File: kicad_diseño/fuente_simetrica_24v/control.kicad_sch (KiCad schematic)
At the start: 6 parts, among them J4 Conn_01x04_Socket, SW1 SW_Push, SW2 SW_Push, U6 ESP32-WROOM-32E, U7 AMS1117-3.3

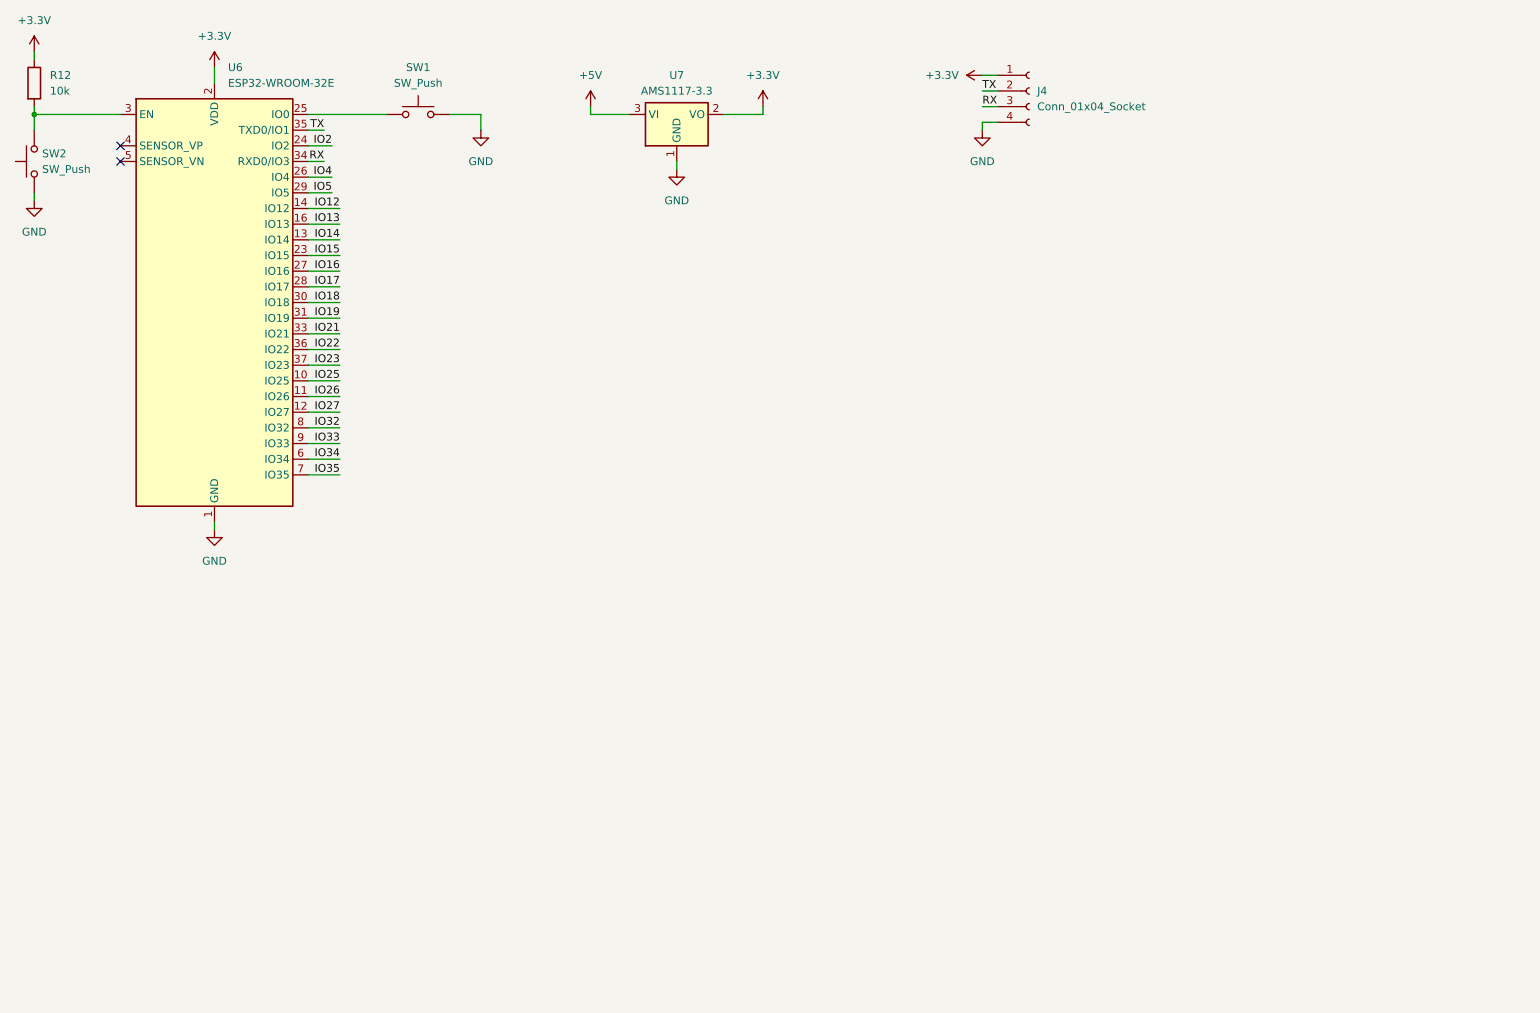
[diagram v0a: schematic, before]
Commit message: Update Fte - Pcb
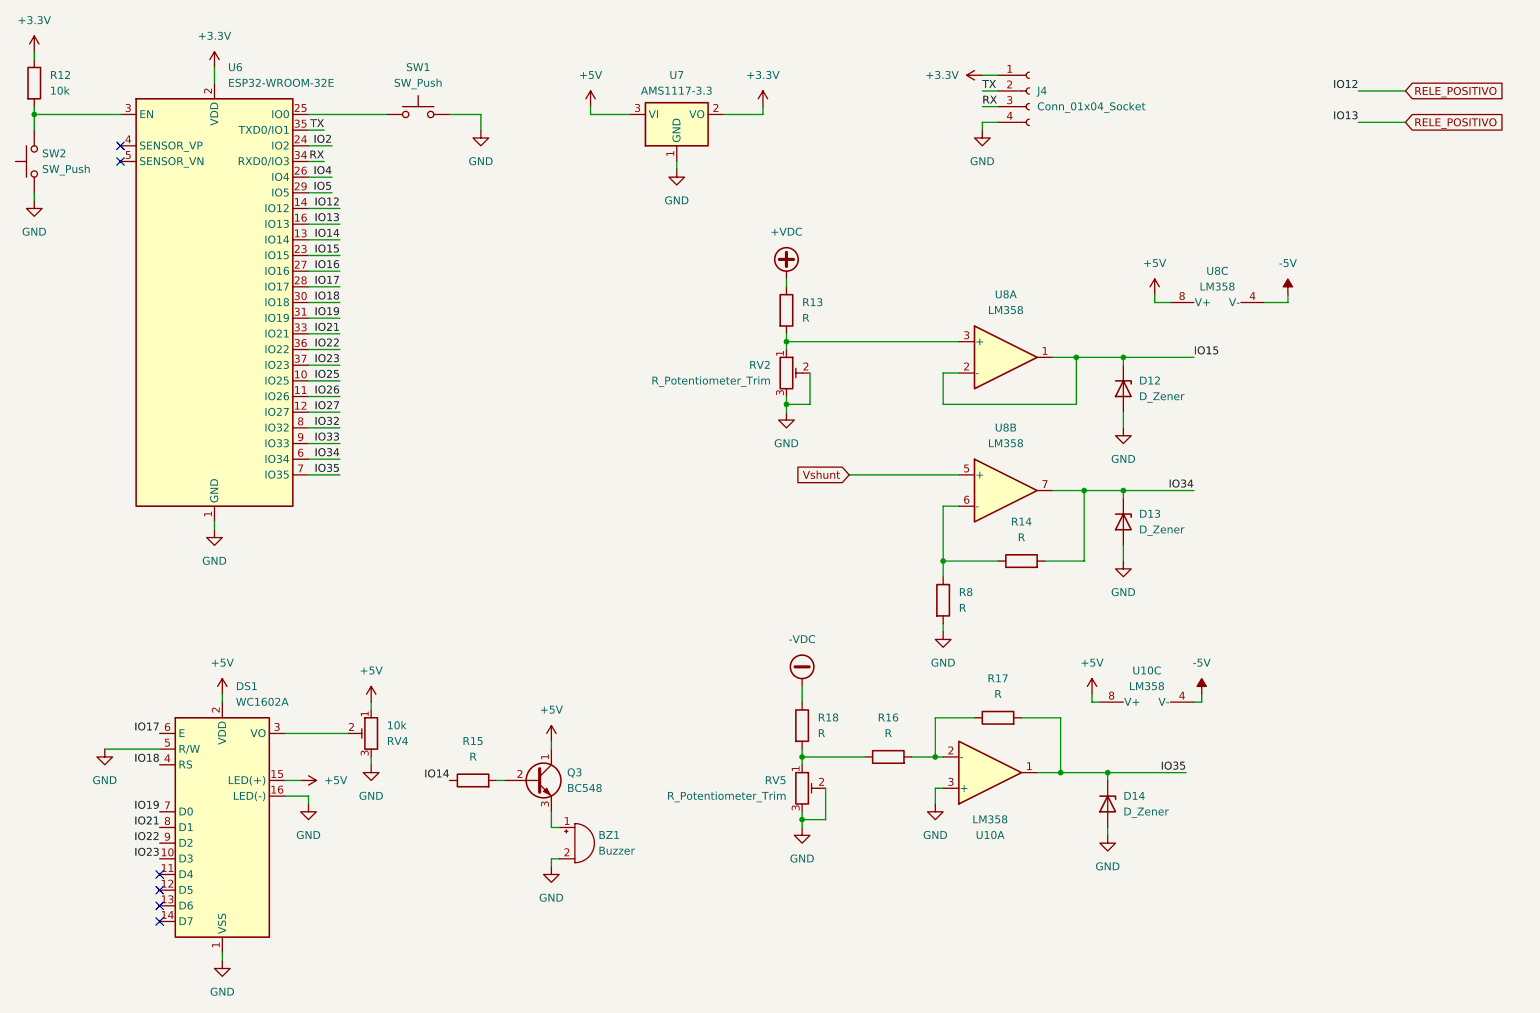
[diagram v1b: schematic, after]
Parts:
- added BZ1: Buzzer, symbol Device:Buzzer
- added D12, D13, D14: D_Zener, symbol Device:D_Zener
- added DS1: WC1602A, Display:WC1602A, symbol Display_Character:WC1602A
- added Q3: BC548, Package_TO_SOT_THT:TO-92_Inline, symbol Transistor_BJT:BC548
- added R13, R14, R15, R16, R17, R18, R8: R, symbol Device:R
- added RV2, RV5: R_Potentiometer_Trim, symbol Device:R_Potentiometer_Trim
- added RV4: 10k, symbol Device:R_Potentiometer_Trim
- added U10, U8: LM358, symbol Amplifier_Operational:LM358
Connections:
- net IO13 is gone; now on net RELE_POSITIVO: U6.16 (IO13)
- net +5V: now also DS1.15 (LED(+)), DS1.2 (VDD), Q3.1 (C), RV4.1, U10.8 (V+), U8.8 (V+)
- net GND: now also BZ1.2 (-), D12.2 (A), D13.2 (A), D14.2 (A), DS1.1 (VSS), DS1.16 (LED(-)), DS1.5 (R/W), R8.2, RV2.2, RV2.3, RV4.3, RV5.2, RV5.3, U10.3 (+)
- net IO14: now also R15.1
- net IO15: now also D12.1 (K), U8.1, U8.2 (-)
- net IO17: now also DS1.6 (E)
- net IO18: now also DS1.4 (RS)
- net IO19: now also DS1.7 (D0)
- net IO21: now also DS1.8 (D1)
- net IO22: now also DS1.9 (D2)
- net IO23: now also DS1.10 (D3)
- net IO34: now also D13.1 (K), R14.2, U8.7
- net IO35: now also D14.1 (K), R17.2, U10.1
- net IO12 renamed RELE_POSITIVO
- new net: R14.1, R8.1, U8.6 (-)
- new net: R16.1, R18.2, RV5.1
- new net: R13.2, RV2.1, U8.3 (+)
- new net: Q3.2 (B), R15.2
- new net: R16.2, R17.1, U10.2 (-)
- new net: BZ1.1 (+), Q3.3 (E)
- new net: DS1.3 (VO), RV4.2
- new net +VDC: R13.1
- new net -5V: U10.4 (V-), U8.4 (V-)
- new net -VDC: R18.1
- new net Vshunt: U8.5 (+)
- no-connect marks 2 -> 6
